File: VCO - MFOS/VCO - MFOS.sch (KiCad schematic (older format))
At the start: 56 parts, among them J1 CV1, J12 RV1P2, J13 RV2P2, J14 RV1P1, J15 RV2P1, J16 RV2P3, J17 RV1P3, J2 CV2, J24 R11_inv, J25 R11_out, J3 CV3, J4 CV4, J5 LIN, J6 SYNC, Q1 SSM2210, Q2 Q_PJFET_DSG, U1 OP275, U2 TL072

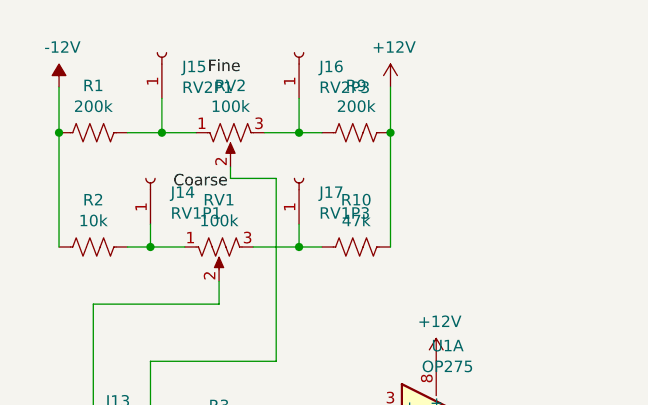
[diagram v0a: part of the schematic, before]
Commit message: literally so much stuff
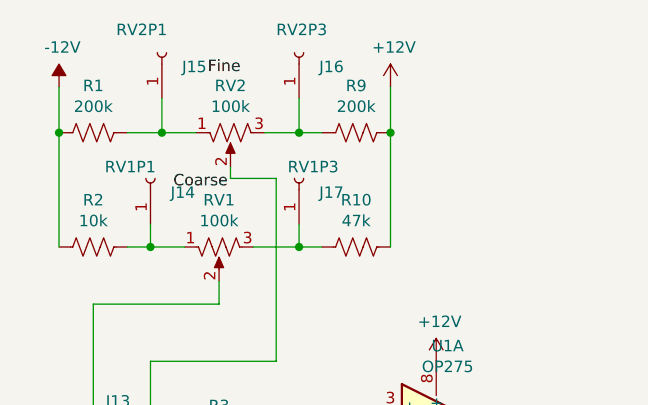
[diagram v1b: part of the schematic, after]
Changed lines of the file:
@@
 P 1500 850
 F 0 "J15" V 1438 762 50  0000 R CNN
-F 1 "RV2P1" V 1347 762 50  0000 R CNN
+F 1 "RV2P1" V 1600 1050 50  0000 R CNN
 F 2 "Connector_Wire:SolderWirePad_1x01_Drill1mm" H 1500 850 50  0001 C CNN
 F 3 "~" H 1500 850 50  0001 C CNN
@@
 P 2100 850
 F 0 "J16" V 2038 762 50  0000 R CNN
-F 1 "RV2P3" V 1947 762 50  0000 R CNN
+F 1 "RV2P3" V 2200 950 50  0000 R CNN
 F 2 "Connector_Wire:SolderWirePad_1x01_Drill1mm" H 2100 850 50  0001 C CNN
 F 3 "~" H 2100 850 50  0001 C CNN
@@
 P 1450 1400
 F 0 "J14" V 1388 1312 50  0000 R CNN
-F 1 "RV1P1" V 1297 1312 50  0000 R CNN
+F 1 "RV1P1" V 1500 1600 50  0000 R CNN
 F 2 "Connector_Wire:SolderWirePad_1x01_Drill1mm" H 1450 1400 50  0001 C CNN
 F 3 "~" H 1450 1400 50  0001 C CNN
@@
 P 2100 1400
 F 0 "J17" V 2038 1312 50  0000 R CNN
-F 1 "RV1P3" V 1947 1312 50  0000 R CNN
+F 1 "RV1P3" V 2150 1450 50  0000 R CNN
 F 2 "Connector_Wire:SolderWirePad_1x01_Drill1mm" H 2100 1400 50  0001 C CNN
 F 3 "~" H 2100 1400 50  0001 C CNN
